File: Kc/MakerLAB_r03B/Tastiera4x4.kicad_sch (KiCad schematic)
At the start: 1 part, among them J27 Conn_01x10_Male

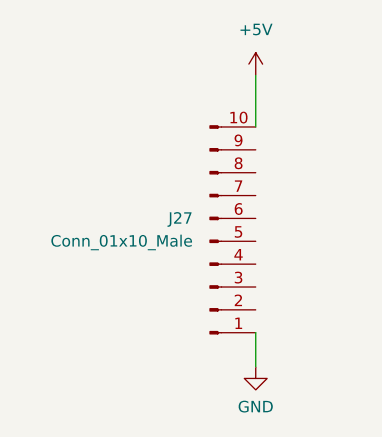
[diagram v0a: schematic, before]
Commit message: versione r03B della notte del 28 marzo 2023
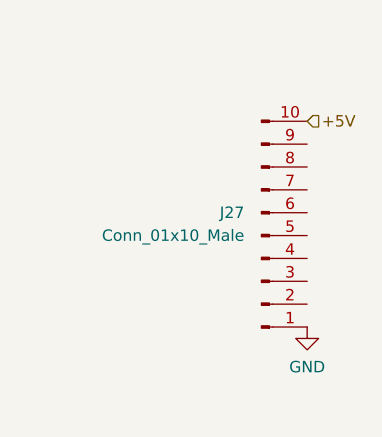
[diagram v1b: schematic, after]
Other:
- moved on the sheet: J27
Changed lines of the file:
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@@
 (kicad_sch (version 20211123) (generator eeschema)
   (paper "A4")
-  (wire (pts (xy 40.005 52.07) (xy 40.005 57.785))
-    (stroke (width 0) (type default) (color 0 0 0 0))
+  (hierarchical_label "+5V" (shape input) (at 45.72 57.15 0)
+    (effects (font (size 1.27 1.27)) (justify left))
   )
-  (wire (pts (xy 40.005 80.645) (xy 40.005 84.455))
-    (stroke (width 0) (type default) (color 0 0 0 0))
-  )
-  (symbol (lib_id "power:GND") (at 40.005 84.455 0) (unit 1)
+  (symbol (lib_id "power:GND") (at 45.72 80.01 0) (unit 1)
     (in_bom yes) (on_board yes) (fields_autoplaced)
-    (property "Reference" "#PWR0103" (id 0) (at 40.005 90.805 0)
+    (property "Reference" "#PWR0103" (id 0) (at 45.72 86.36 0)
       (effects (font (size 1.27 1.27)) hide)
     )
-    (property "Value" "GND" (id 1) (at 40.005 88.9 0))
-    (property "Footprint" "" (id 2) (at 40.005 84.455 0)
+    (property "Value" "GND" (id 1) (at 45.72 84.455 0))
+    (property "Footprint" "" (id 2) (at 45.72 80.01 0)
       (effects (font (size 1.27 1.27)) hide)
     )
-    (property "Datasheet" "" (id 3) (at 40.005 84.455 0)
+    (property "Datasheet" "" (id 3) (at 45.72 80.01 0)
       (effects (font (size 1.27 1.27)) hide)
     )
     (pin "1")
   )
-  (symbol (lib_id "Connector:Conn_01x10_Male") (at 34.925 70.485 0) (mirror x) (unit 1)
+  (symbol (lib_id "Connector:Conn_01x10_Male") (at 40.64 69.85 0) (mirror x) (unit 1)
     (in_bom yes) (on_board yes) (fields_autoplaced)
-    (property "Reference" "J27" (id 0) (at 33.02 67.9449 0)
+    (property "Reference" "J27" (id 0) (at 38.735 67.3099 0)
       (effects (font (size 1.27 1.27)) (justify right))
     )
-    (property "Value" "Conn_01x10_Male" (id 1) (at 33.02 70.4849 0)
+    (property "Value" "Conn_01x10_Male" (id 1) (at 38.735 69.8499 0)
       (effects (font (size 1.27 1.27)) (justify right))
     )
-    (property "Footprint" "" (id 2) (at 34.925 70.485 0)
+    (property "Footprint" "" (id 2) (at 40.64 69.85 0)
       (effects (font (size 1.27 1.27)) hide)
     )
-    (property "Datasheet" "~" (id 3) (at 34.925 70.485 0)
+    (property "Datasheet" "~" (id 3) (at 40.64 69.85 0)
       (effects (font (size 1.27 1.27)) hide)
     )
@@
     (pin "9")
   )
-  (symbol (lib_id "power:+5V") (at 40.005 52.07 0) (unit 1)
-    (in_bom yes) (on_board yes) (fields_autoplaced)
-    (property "Reference" "#PWR0104" (id 0) (at 40.005 55.88 0)
-      (effects (font (size 1.27 1.27)) hide)
-    )
-    (property "Value" "+5V" (id 1) (at 40.005 46.99 0))
-    (property "Footprint" "" (id 2) (at 40.005 52.07 0)
-      (effects (font (size 1.27 1.27)) hide)
-    )
-    (property "Datasheet" "" (id 3) (at 40.005 52.07 0)
-      (effects (font (size 1.27 1.27)) hide)
-    )
-    (pin "1")
-  )
 )
